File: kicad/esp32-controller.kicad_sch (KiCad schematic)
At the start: 26 parts, among them J1 Conn_01x08_Socket, Q1 BCW66G, Q2 BCW66G, SW1 RESET, SW2 BOOT, U1 ESP32-WROVER-IB, U2 PS4, U3 PS4, U4 CH340C

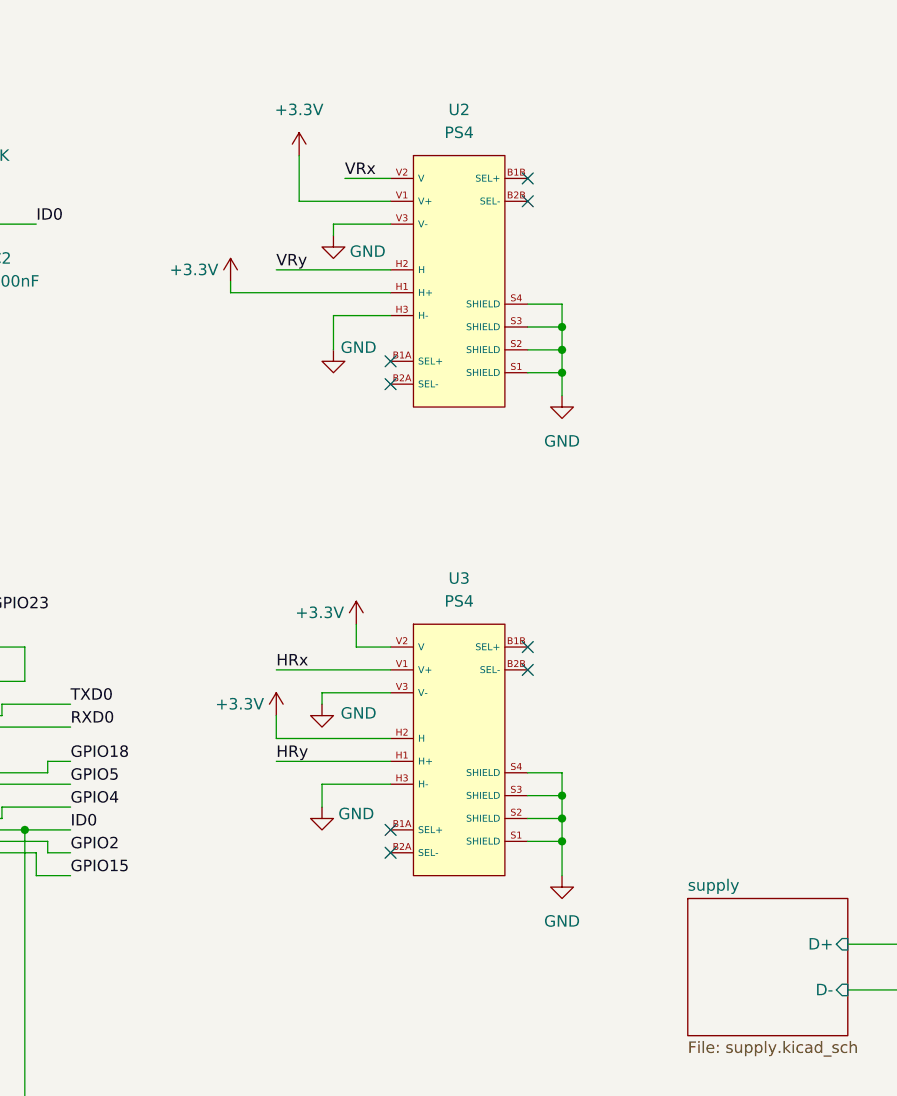
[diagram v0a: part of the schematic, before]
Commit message: init
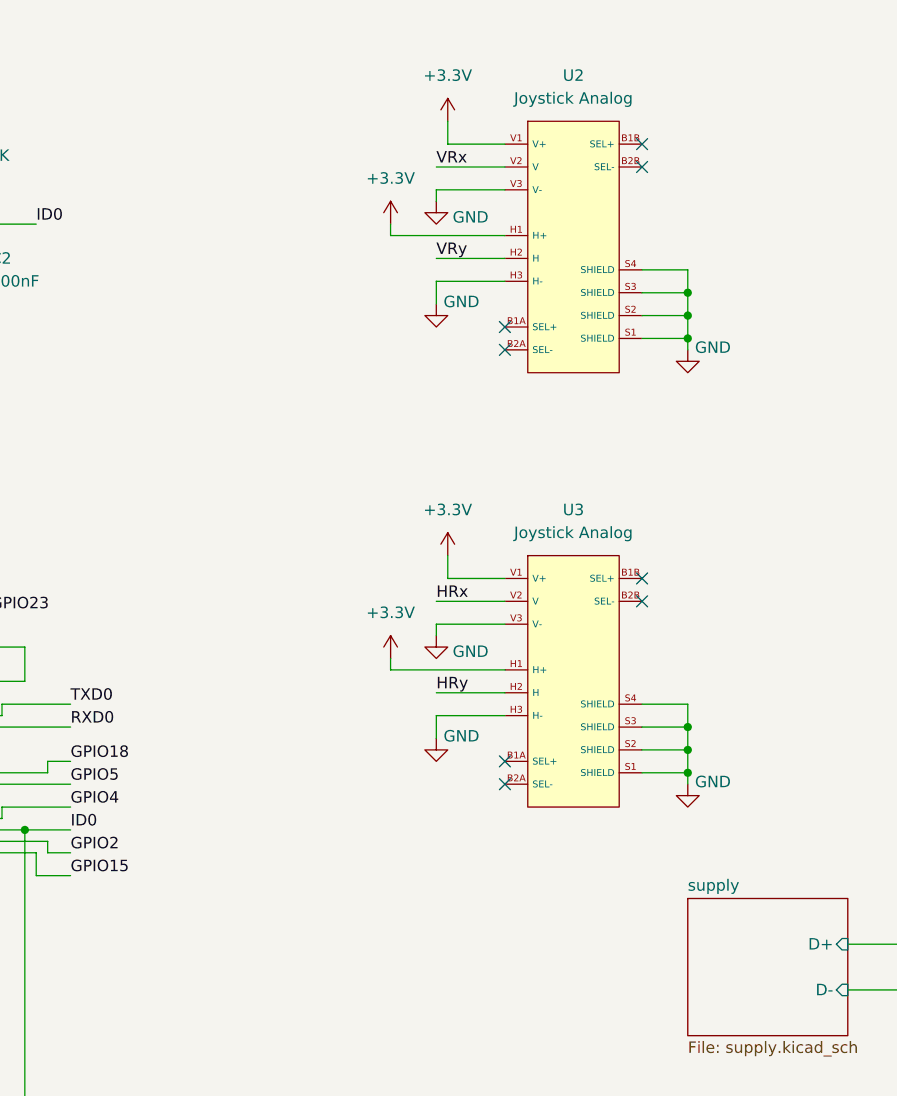
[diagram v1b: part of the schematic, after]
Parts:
- removed U2, U3: PS4, PCM_yvolodym:Joystick_PS5, symbol PCM_yvolodym:Joystick_PS5
- added U2, U3: Joystick Analog, PCM_yvolodym:Joystick_Analog, symbol PCM_yvolodym:Joystick_Analog
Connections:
- net +3.3V: now also U2.H1 (H+), U2.V1 (V+), U3.H1 (H+), U3.V1 (V+)
- net GND: now also U2.H3 (H-), U2.S1 (SHIELD), U2.S2 (SHIELD), U2.S3 (SHIELD), U2.S4 (SHIELD), U2.V3 (V-), U3.H3 (H-), U3.S1 (SHIELD), U3.S2 (SHIELD), U3.S3 (SHIELD), U3.S4 (SHIELD), U3.V3 (V-)
- net HRx: now also U3.V2 (V)
- net HRy: now also U3.H2 (H)
- net VRx: now also U2.V2 (V)
- net VRy: now also U2.H2 (H)
